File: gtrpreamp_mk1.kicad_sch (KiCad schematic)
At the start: 114 parts, among them Q1 2N5457, Q2 2N5457, U1 NE5532, U2 NE5532, U3 NE5532, U4 L78L09_TO92

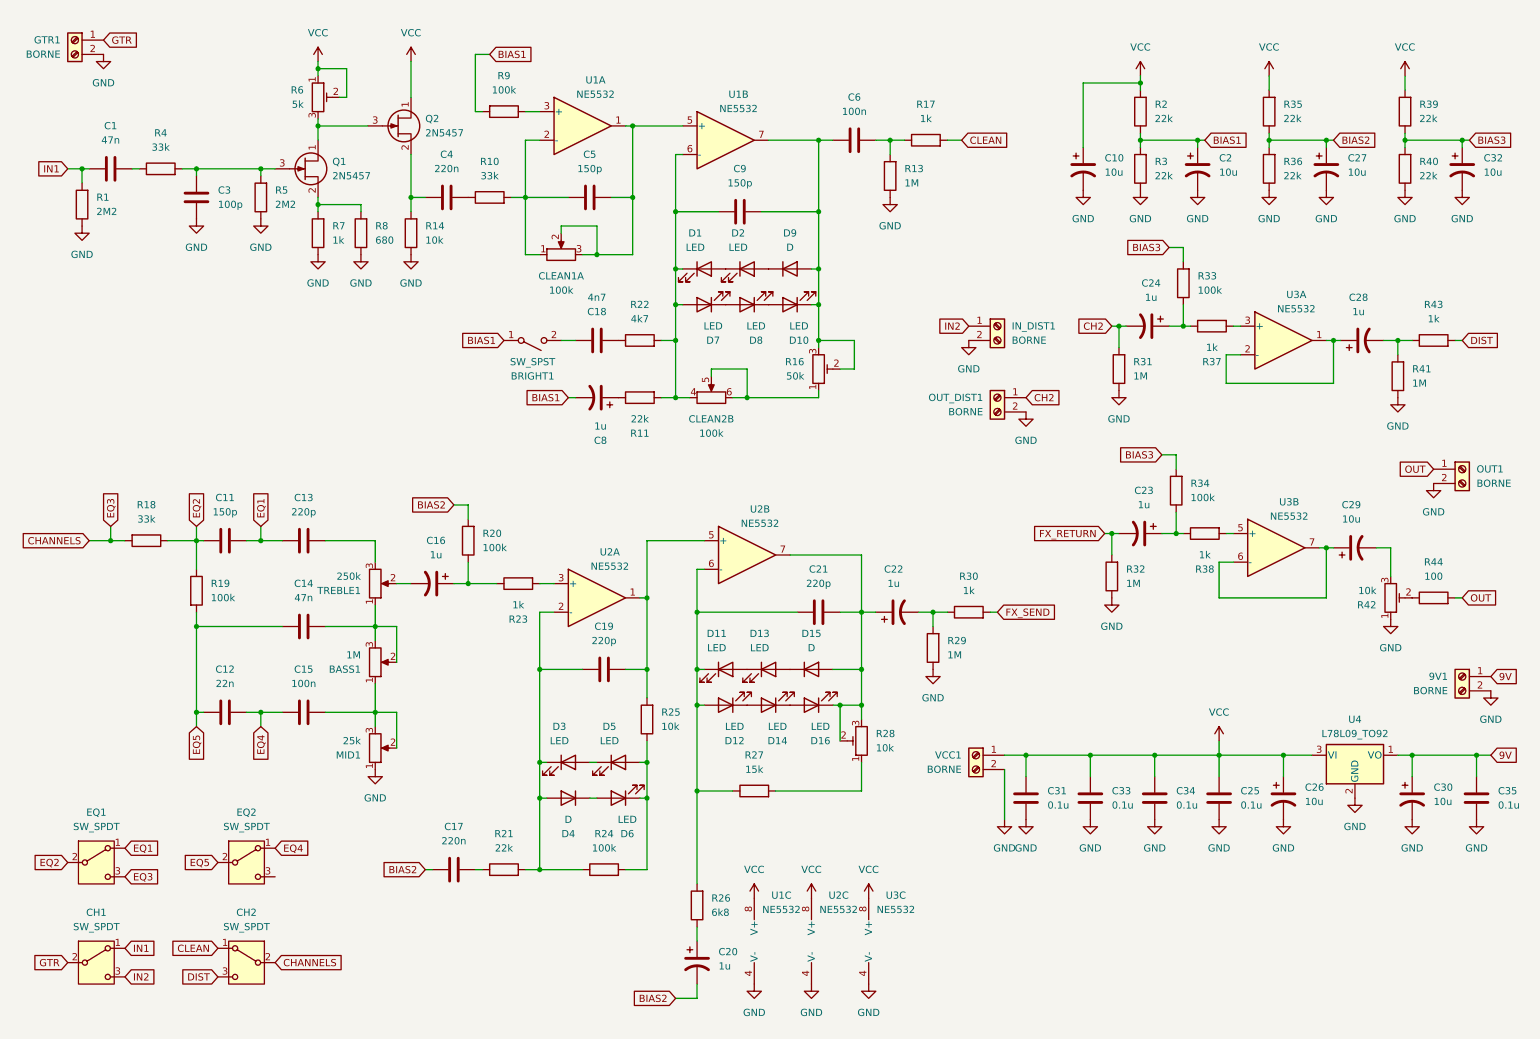
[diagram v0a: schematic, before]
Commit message: modifico etapas
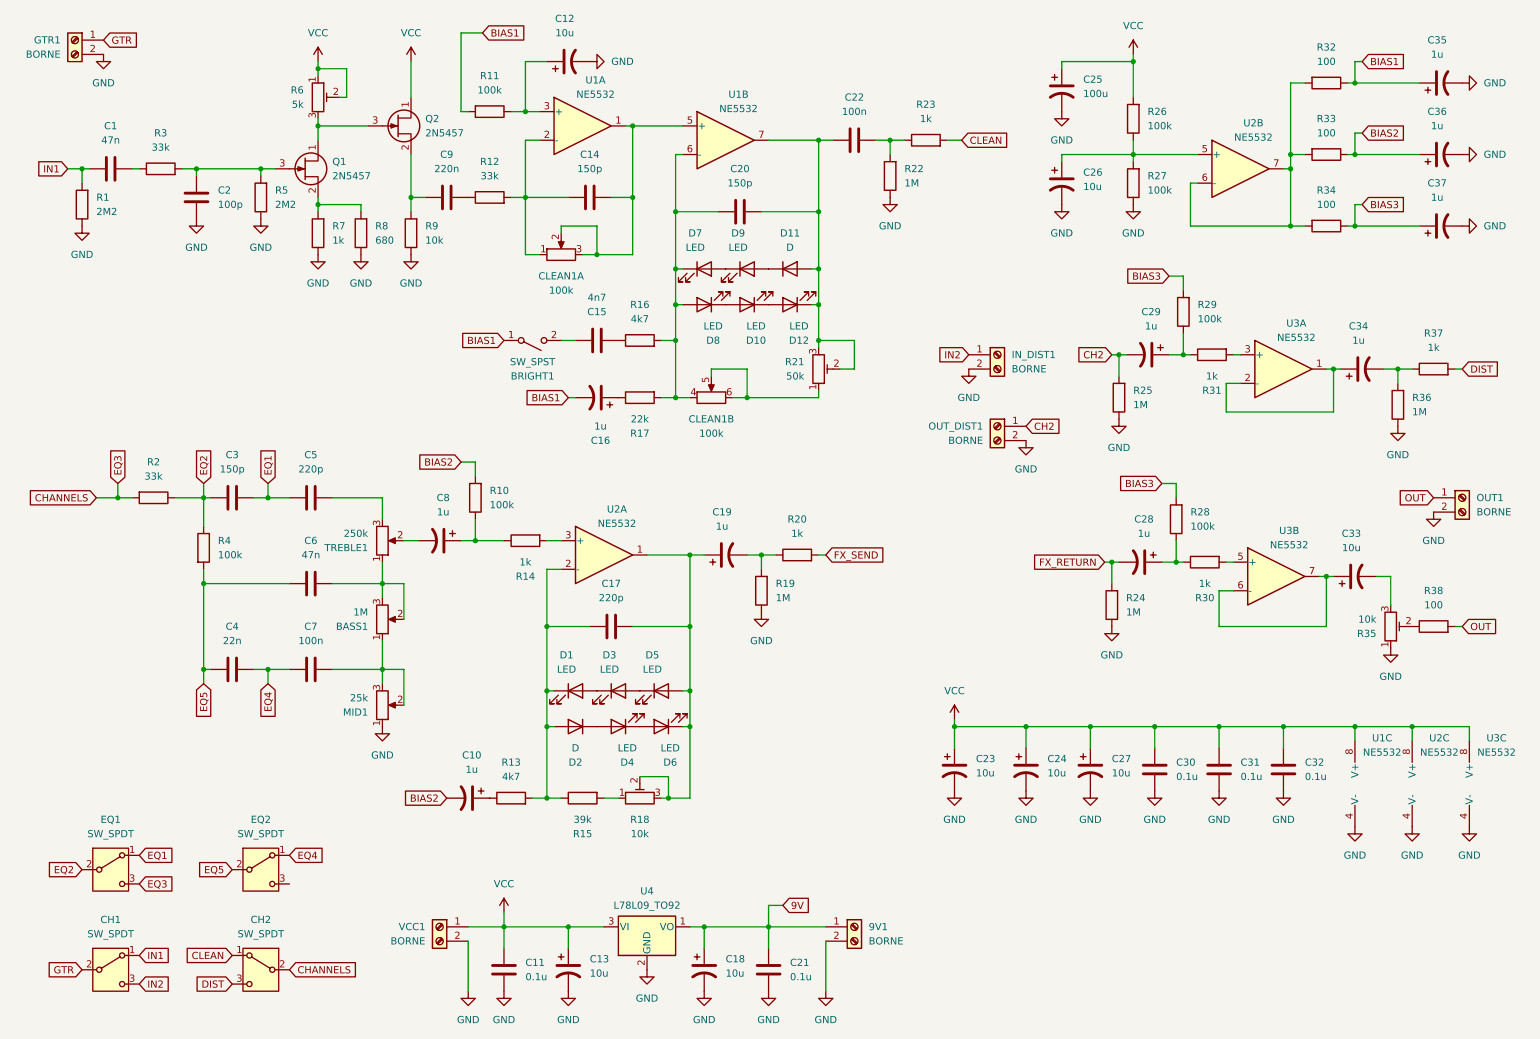
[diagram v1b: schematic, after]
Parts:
- removed C17: 220n, Capacitor_THT:C_Rect_L9.0mm_W4.0mm_P7.50mm_MKT, symbol Device:C
- removed C2, C32: 10u, Capacitor_THT:CP_Radial_D6.3mm_P2.50mm, symbol Device:C_Polarized_US
- removed C21: 220p, Capacitor_THT:C_Disc_D5.0mm_W2.5mm_P5.00mm, symbol Device:C
- removed D11, D12, D13, D14, D16: LED, LED_THT:LED_D3.0mm_Clear, symbol Device:LED
- removed D15: D, symbol Device:D
- removed R25: 10k, Resistor_THT:R_Axial_DIN0207_L6.3mm_D2.5mm_P7.62mm_Horizontal, symbol Device:R
- removed R26: 6k8, Resistor_THT:R_Axial_DIN0207_L6.3mm_D2.5mm_P7.62mm_Horizontal, symbol Device:R
- removed R27: 15k, Resistor_THT:R_Axial_DIN0207_L6.3mm_D2.5mm_P7.62mm_Horizontal, symbol Device:R
- removed R35, R36, R39, R40: 22k, Resistor_THT:R_Axial_DIN0207_L6.3mm_D2.5mm_P7.62mm_Horizontal, symbol Device:R
- added C12, C23, C24, C26: 10u, Capacitor_THT:CP_Radial_D6.3mm_P2.50mm, symbol Device:C_Polarized_US
- added C35, C36, C37: 1u, Capacitor_THT:CP_Radial_D6.3mm_P2.50mm, symbol Device:C_Polarized_US
- added D5, D6: LED, LED_THT:LED_D3.0mm_Clear, symbol Device:LED
- added R32, R33, R34: 100, Resistor_THT:R_Axial_DIN0207_L6.3mm_D2.5mm_P7.62mm_Horizontal, symbol Device:R
- C25: renamed from C10; value 10u -> 100u
- R13: renamed from R21; value 22k -> 4k7
- R15: renamed from R24; value 100k -> 39k
- R26: renamed from R2; value 22k -> 100k
- R27: renamed from R3; value 22k -> 100k
- renumbered C20 to C10, C25 to C11, C26 to C13, C5 to C14, C18 to C15, C8 to C16, C19 to C17, C30 to C18, C22 to C19, C3 to C2, C9 to C20, C35 to C21, C6 to C22, C23 to C28, C24 to C29, C11 to C3, C31 to C30, C33 to C31, C34 to C32, C29 to C33, C28 to C34, C12 to C4, C13 to C5, C14 to C6, C15 to C7, C16 to C8, C4 to C9, CLEAN2 to CLEAN1, D3 to D1, D8 to D10, D9 to D11, D10 to D12, D4 to D2, D5 to D3, D6 to D4, D1 to D7, D7 to D8, D2 to D9, R20 to R10, R9 to R11, R10 to R12, R23 to R14, R22 to R16, R11 to R17, R28 to R18, R29 to R19, R18 to R2, R30 to R20, R16 to R21, R13 to R22, R17 to R23, R32 to R24, R31 to R25, R34 to R28, R33 to R29, R4 to R3, R38 to R30, R37 to R31, R42 to R35, R41 to R36, R43 to R37, R44 to R38, R19 to R4, R14 to R9
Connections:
- net BIAS1: now also C35.1, R32.1; no longer R26.1, R27.2
- net BIAS2: now also C36.1, R33.1; no longer C27.1
- net BIAS3: now also C37.1, R34.1
- net GND: now also C12.2, C23.2, C24.2, C26.2, C35.2, C36.2, C37.2
- net VCC: now also C27.1, C23.1, C24.1
- net at R18.1: now also R15.2
- net at C19.1, R18.2, R18.3: now also C17.2, U2.1, D5.2 (A), D6.1 (K); no longer U2.7
- net at U2.6 (-): now also U2.7, R32.2, R33.2, R34.2
- net at R11.1, U1.3 (+): now also C12.1
- net at C10.1: now also R13.1
- new net: C26.1, R26.1, R27.2, U2.5 (+)
- new net: D4.1 (K), D6.2 (A)
- new net: D3.2 (A), D5.1 (K)
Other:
- moved on the sheet: 9V1, BASS1, C10, C11, C13, C17, C18, C19, C21, C25, C28, C29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
